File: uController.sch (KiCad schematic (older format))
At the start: 17 parts

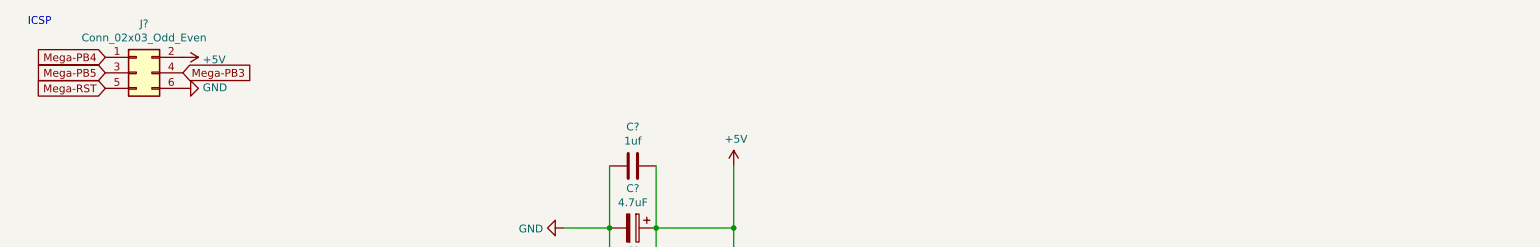
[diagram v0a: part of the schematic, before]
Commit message: updates
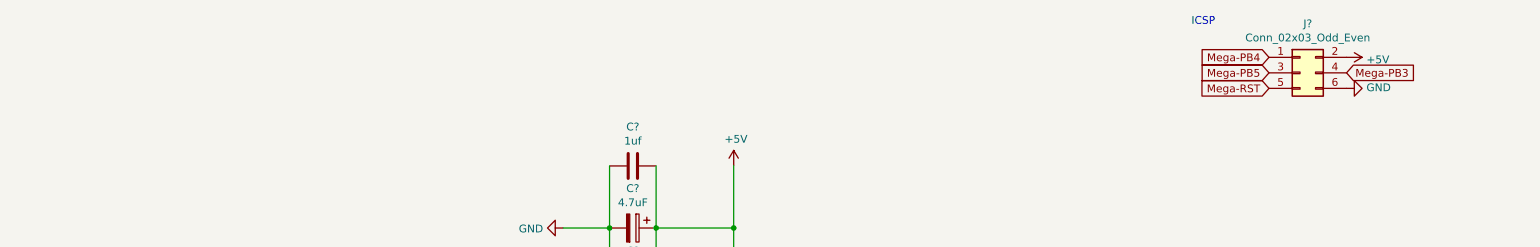
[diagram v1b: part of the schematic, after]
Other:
- moved on the sheet: J?
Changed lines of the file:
@@
 Text Notes 8350 3800 0    50   ~ 0
 CLOCK
-Text Notes 1000 1000 0    50   ~ 0
+Text Notes 8500 1000 0    50   ~ 0
 ICSP
 $Comp
@@
 L Connector_Generic:Conn_02x03_Odd_Even J?
 U 1 1 60E96908
-P 1700 1300
+P 9200 1300
 AR Path="/60E96908" Ref="J?"  Part="1"
 AR Path="/60E76DCE/60E96908" Ref="J?"  Part="1"
-F 0 "J?" H 1750 1617 50  0000 C CNN
-F 1 "Conn_02x03_Odd_Even" H 1750 1526 50  0000 C CNN
-F 2 "" H 1700 1300 50  0001 C CNN
-F 3 "~" H 1700 1300 50  0001 C CNN
-	1    1700 1300
+F 0 "J?" H 9250 1617 50  0000 C CNN
+F 1 "Conn_02x03_Odd_Even" H 9250 1526 50  0000 C CNN
+F 2 "" H 9200 1300 50  0001 C CNN
+F 3 "~" H 9200 1300 50  0001 C CNN
+	1    9200 1300
 	1    0    0    -1
 $EndComp
@@
 L power:GND #PWR?
 U 1 1 60E9690E
-P 2000 1400
+P 9500 1400
 AR Path="/60E9690E" Ref="#PWR?"  Part="1"
 AR Path="/60E76DCE/60E9690E" Ref="#PWR?"  Part="1"
-F 0 "#PWR?" H 2000 1150 50  0001 C CNN
-F 1 "GND" V 2005 1272 50  0000 R CNN
-F 2 "" H 2000 1400 50  0001 C CNN
-F 3 "" H 2000 1400 50  0001 C CNN
-	1    2000 1400
+F 0 "#PWR?" H 9500 1150 50  0001 C CNN
+F 1 "GND" V 9505 1272 50  0000 R CNN
+F 2 "" H 9500 1400 50  0001 C CNN
+F 3 "" H 9500 1400 50  0001 C CNN
+	1    9500 1400
 	0    -1   -1   0
 $EndComp
@@
 L power:+5V #PWR?
 U 1 1 60E96914
-P 2000 1200
+P 9500 1200
 AR Path="/60E96914" Ref="#PWR?"  Part="1"
 AR Path="/60E76DCE/60E96914" Ref="#PWR?"  Part="1"
-F 0 "#PWR?" H 2000 1050 50  0001 C CNN
-F 1 "+5V" V 2015 1328 50  0000 L CNN
-F 2 "" H 2000 1200 50  0001 C CNN
-F 3 "" H 2000 1200 50  0001 C CNN
-	1    2000 1200
+F 0 "#PWR?" H 9500 1050 50  0001 C CNN
+F 1 "+5V" V 9515 1328 50  0000 L CNN
+F 2 "" H 9500 1200 50  0001 C CNN
+F 3 "" H 9500 1200 50  0001 C CNN
+	1    9500 1200
 	0    1    1    0
 $EndComp
-Text GLabel 2000 1300 2    50   Input ~ 0
+Text GLabel 9500 1300 2    50   Input ~ 0
 Mega-PB3
-Text GLabel 1500 1400 0    50   Input ~ 0
+Text GLabel 9000 1400 0    50   Input ~ 0
 Mega-RST
-Text GLabel 1500 1300 0    50   Input ~ 0
+Text GLabel 9000 1300 0    50   Input ~ 0
 Mega-PB5
-Text GLabel 1500 1200 0    50   Input ~ 0
+Text GLabel 9000 1200 0    50   Input ~ 0
 Mega-PB4
 $Comp
